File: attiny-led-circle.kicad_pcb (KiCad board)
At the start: 2 copper layers, 50.8 x 50.8 mm, 15 parts, among them J1 USB_B_Micro, U1 ATtiny13A-PU

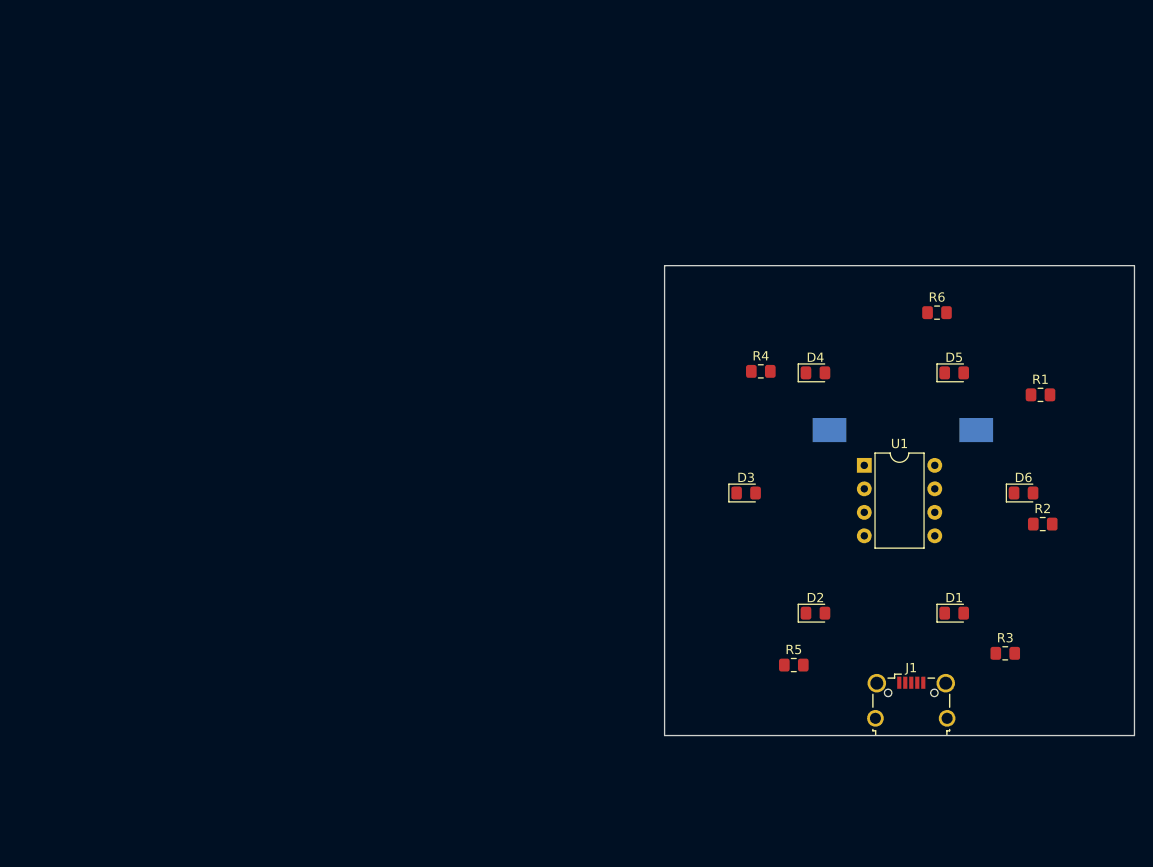
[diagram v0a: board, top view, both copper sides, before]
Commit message: Update
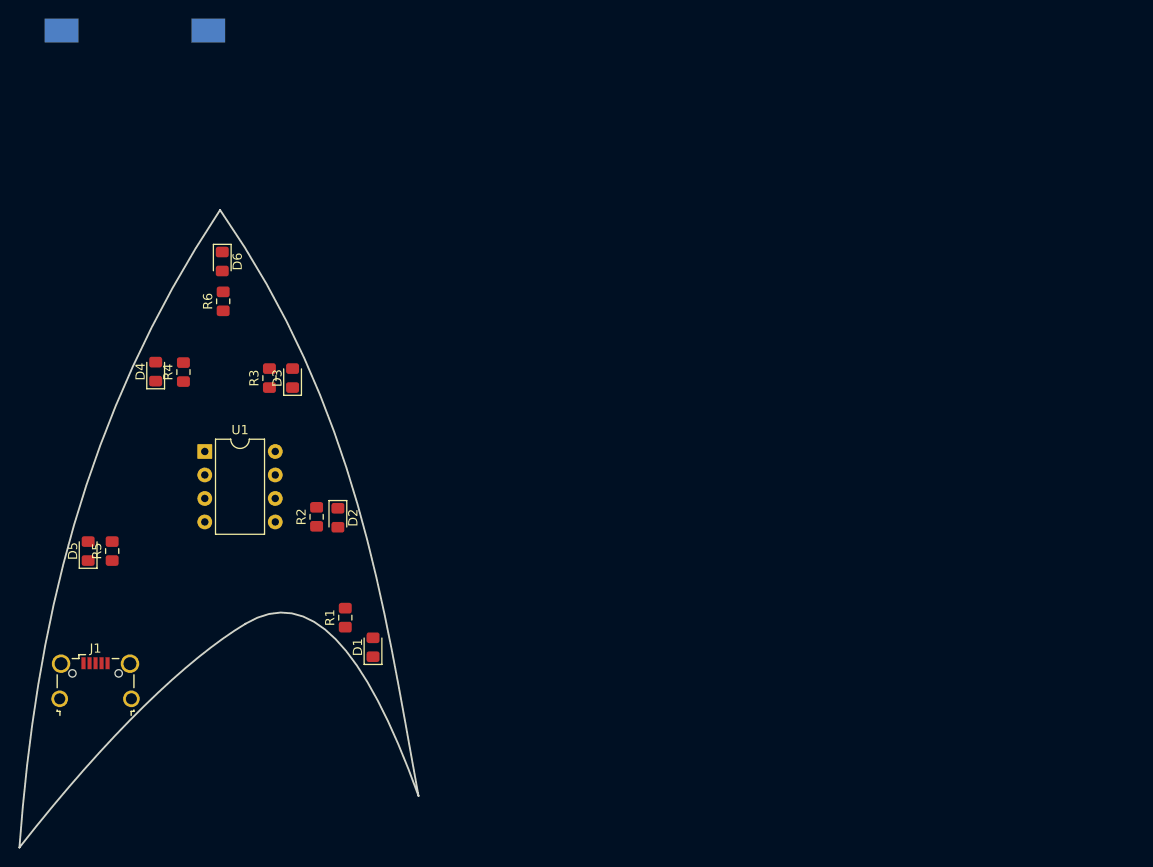
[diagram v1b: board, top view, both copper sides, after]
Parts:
- moved D5 95.6 mm to (59.6, 89.3), turned to 90 degrees
- moved BT1 93.6 mm to (64.3, 33.0)
- moved D6 90.2 mm to (74.1, 58.0), turned to 270 degrees
- moved J1 88.2 mm to (60.4, 103.3)
- moved R3 84.9 mm to (79.2, 70.6), turned to 90 degrees
- moved R1 78.9 mm to (87.4, 96.5), turned to 90 degrees
- moved R2 78.5 mm to (84.3, 85.6), turned to 90 degrees
- moved R6 77.2 mm to (74.2, 62.3), turned to 90 degrees
- moved R5 74.7 mm to (62.2, 89.3), turned to 90 degrees
- moved D4 71.3 mm to (66.9, 69.9), turned to 90 degrees
- moved U1 71.3 mm to (72.2, 78.5)
- moved D1 62.9 mm to (90.4, 99.7), turned to 90 degrees
- moved R4 62.4 mm to (69.9, 69.9), turned to 90 degrees
- moved D2 52.7 mm to (86.6, 85.7), turned to 270 degrees
- moved D3 50.6 mm to (81.7, 70.6), turned to 90 degrees
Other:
- board size 50.8 x 50.8 mm -> 43.1 x 68.9 mm
